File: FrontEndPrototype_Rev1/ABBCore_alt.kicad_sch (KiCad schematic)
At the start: 20 parts, among them J10 MIllMaxSpringConnector, J3 MIllMaxSpringConnector, J4 MIllMaxSpringConnector, J5 MIllMaxSpringConnector, J6 MIllMaxSpringConnector, J7 MIllMaxSpringConnector, J8 MIllMaxSpringConnector, J9 MIllMaxSpringConnector, U1 CD74AC238, U2 ADA4807-2ACP

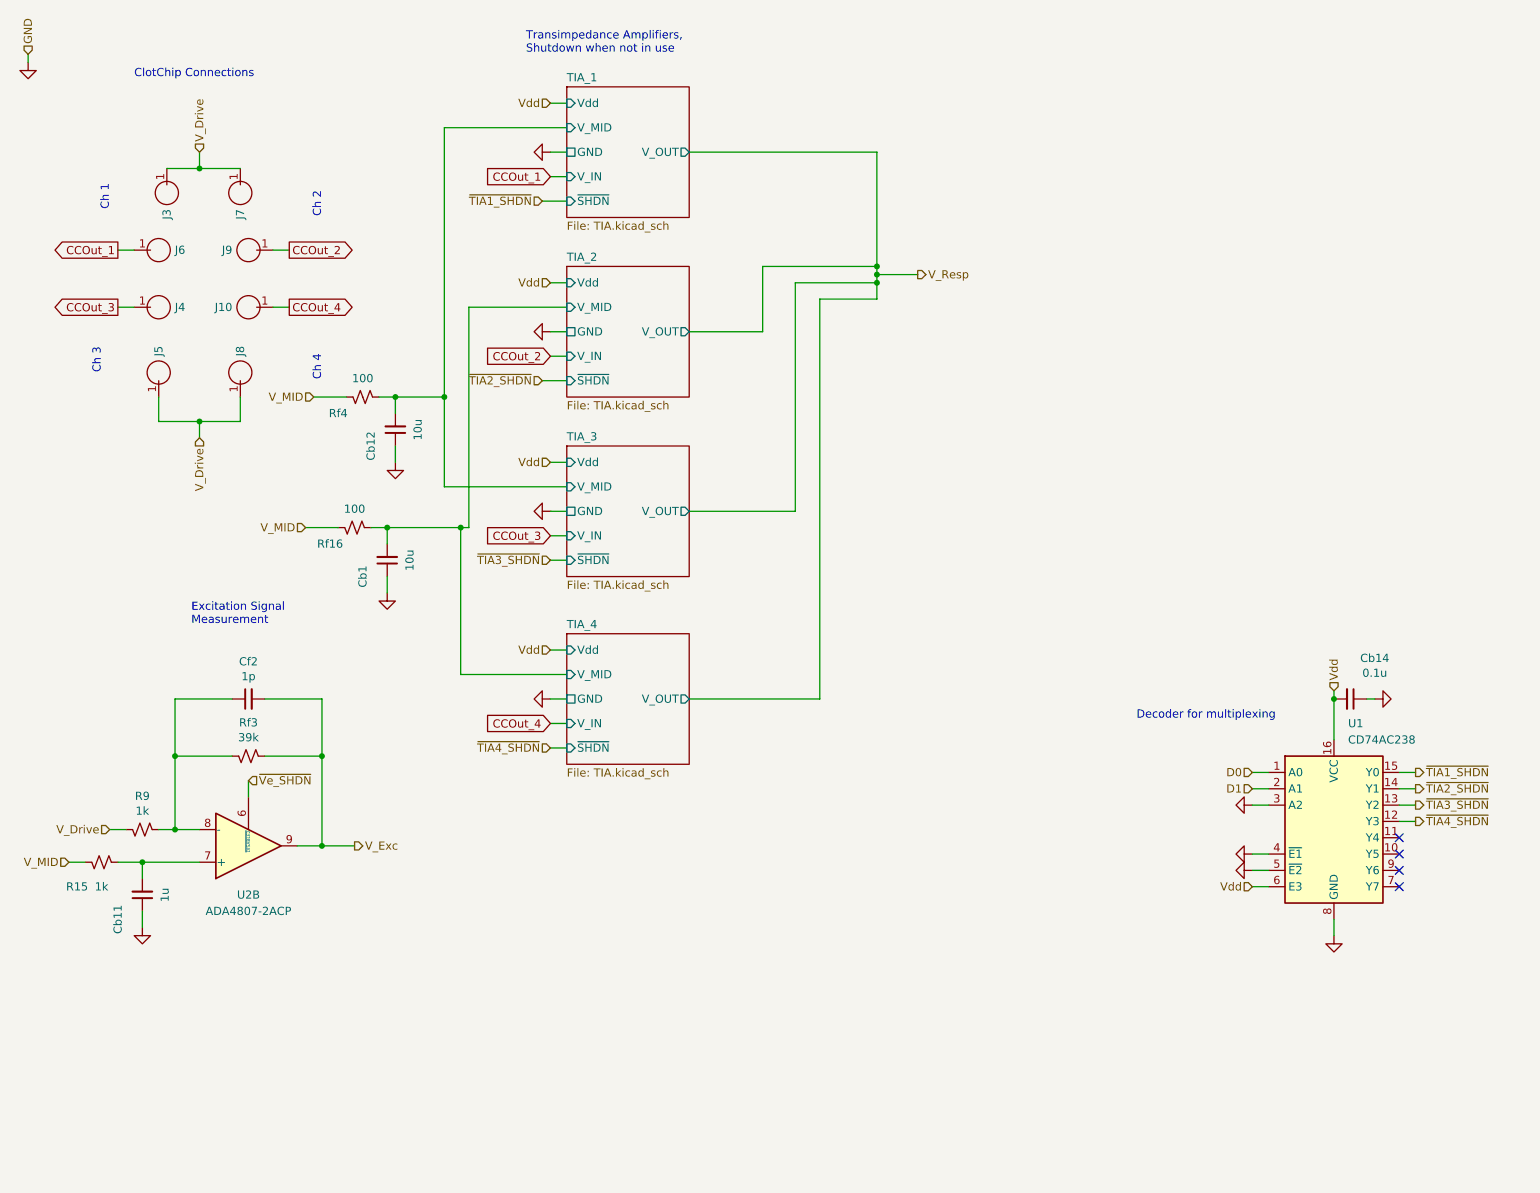
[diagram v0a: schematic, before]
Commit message: First Pass Schematic Fixes for Power Management Board
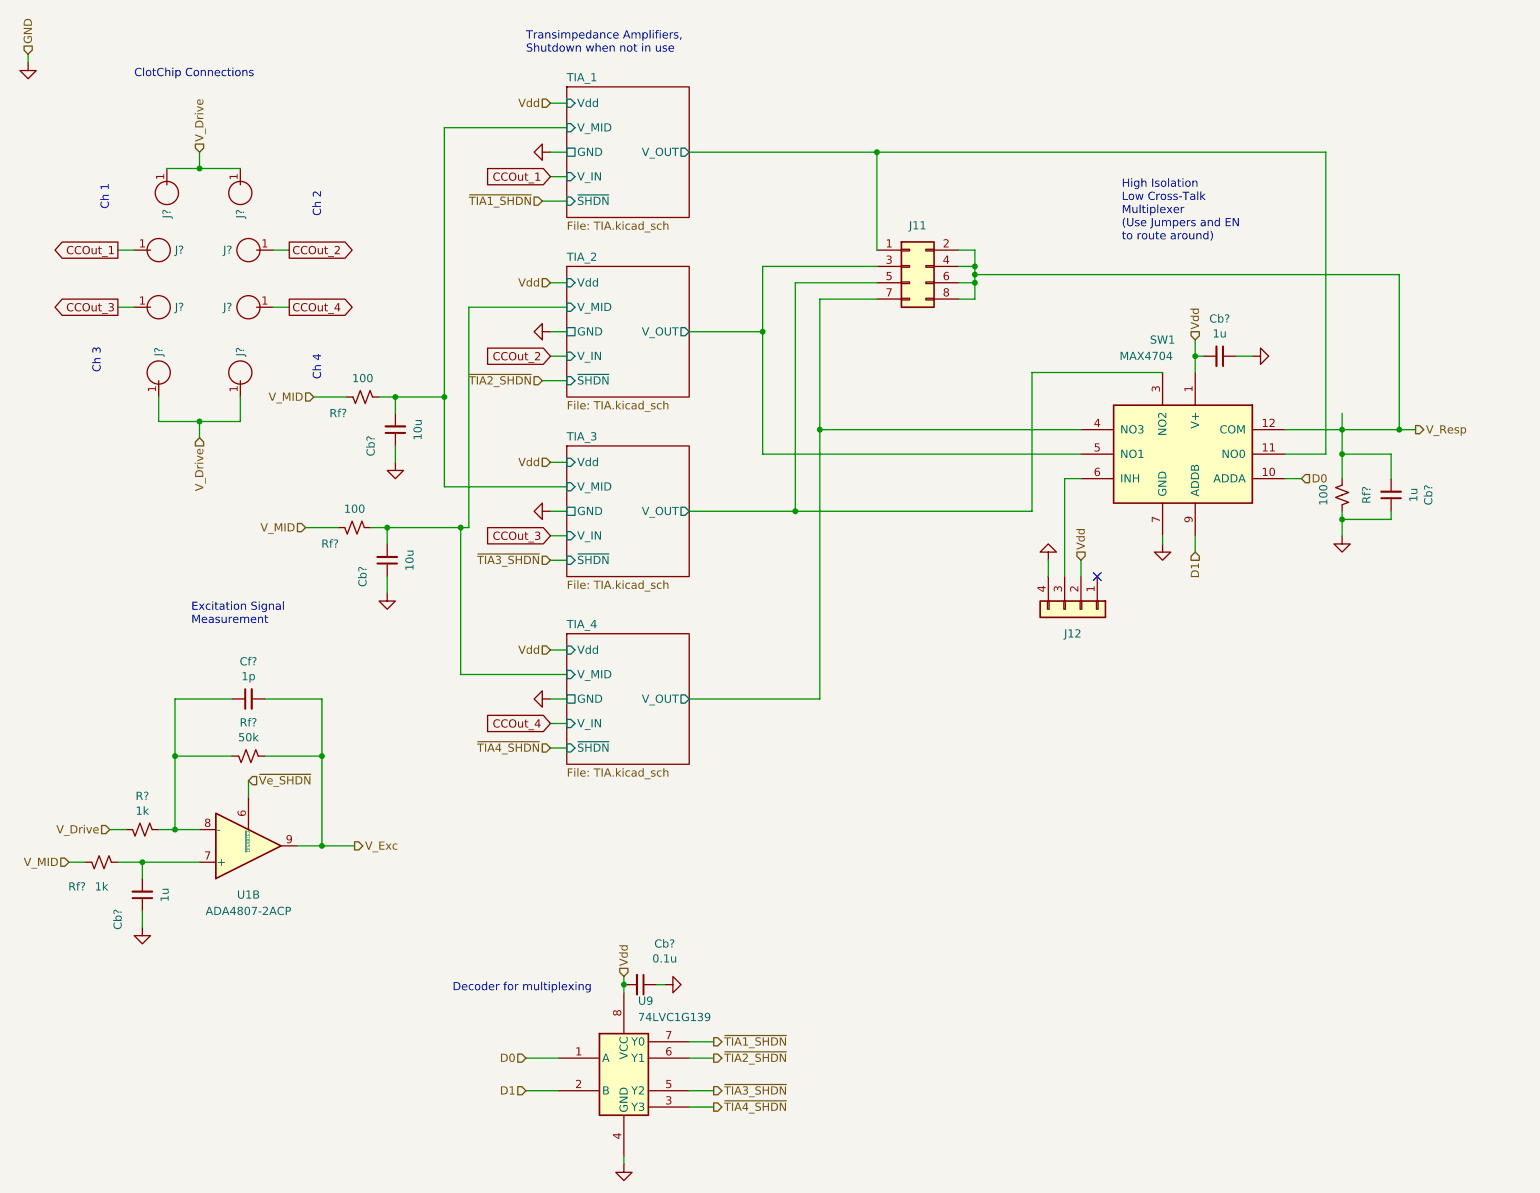
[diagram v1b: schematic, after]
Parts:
- removed Cb14: 0.1u, Capacitor_SMD:C_0603_1608Metric_Pad1.08x0.95mm_HandSolder, symbol Device:C_Small
- removed U1: CD74AC238, Package_SO:TSSOP-16_4.4x5mm_P0.65mm, symbol 74xx:CD74AC238
- added Cb? (x2): 1u, Capacitor_SMD:C_0603_1608Metric_Pad1.08x0.95mm_HandSolder, symbol Device:C_Small
- added Cb?: 0.1u, Capacitor_SMD:C_0603_1608Metric_Pad1.08x0.95mm_HandSolder, symbol Device:C_Small
- added J11: Conn_02x04_Odd_Even, Connector_PinHeader_2.54mm:PinHeader_2x04_P2.54mm_Vertical_SMD, symbol Connector_Generic:Conn_02x04_Odd_Even
- added J12: Conn_02x02_Odd_Even, Connector_PinHeader_2.54mm:PinHeader_1x04_P2.54mm_Vertical_SMD_Pin1Right, symbol Connector_Generic:Conn_01x04
- added Rf?: 100, Resistor_SMD:R_0603_1608Metric_Pad0.98x0.95mm_HandSolder, symbol Device:R_Small_US
- added SW1: MAX4704, Package_DFN_QFN:DFN-12-1EP_3x3mm_P0.5mm_EP1.6x2.5mm, symbol FrontEndPrototype_Rev1-rescue:MAX4704
- added U9: 74LVC1G139, Package_SO:VSSOP-8_2.3x2mm_P0.5mm, symbol 74xGxx:74LVC1G139
- Rf?: renamed from Rf3; value 39k -> 50k
- renumbered Cb11 to Cb?, Cb12 to Cb?, Cb1 to Cb?, Cf2 to Cf?, J9 to J?, J3 to J?, J7 to J?, J5 to J?, J6 to J?, J8 to J?, J10 to J?, J4 to J?, R9 to R?, R15 to Rf?, Rf4 to Rf?, Rf16 to Rf?, U2 to U1
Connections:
- net D0: now also SW1.10 (ADDA), U9.1 (A)
- net D1: now also SW1.9 (ADDB), U9.2 (B)
- net GND: now also Cb?.1, Cb?.1, Cb?.1, J12.4 (Pin_4), Rf?.1, SW1.7 (GND), U9.4 (GND)
- net V_Resp: now also Cb?.2, J11.2 (Pin_2), J11.4 (Pin_4), J11.6 (Pin_6), J11.8 (Pin_8), Rf?.2, SW1.12 (COM)
- net Vdd: now also Cb?.2, Cb?.2, J12.2 (Pin_2), SW1.1 (V+), U9.8 (VCC)
- net ~{TIA1_SHDN}: now also U9.7 (Y0)
- net ~{TIA2_SHDN}: now also U9.6 (Y1)
- net ~{TIA3_SHDN}: now also U9.5 (Y2)
- net ~{TIA4_SHDN}: now also U9.3 (Y3)
- new net: J12.3 (Pin_3), SW1.6 (INH)
- new net TIA_1/V_OUT: J11.1 (Pin_1), SW1.11 (NO0)
- new net TIA_2/V_OUT: J11.3 (Pin_3), SW1.5 (NO1)
- new net TIA_3/V_OUT: J11.5 (Pin_5), SW1.3 (NO2)
- new net TIA_4/V_OUT: J11.7 (Pin_7), SW1.4 (NO3)
- no-connect marks 4 -> 1
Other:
- note added: "High Isolation Low Cross-Talk Multiplexer (Use Jumpers and EN to route around)"

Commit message: Updated Measurement Board with new 3V Reference
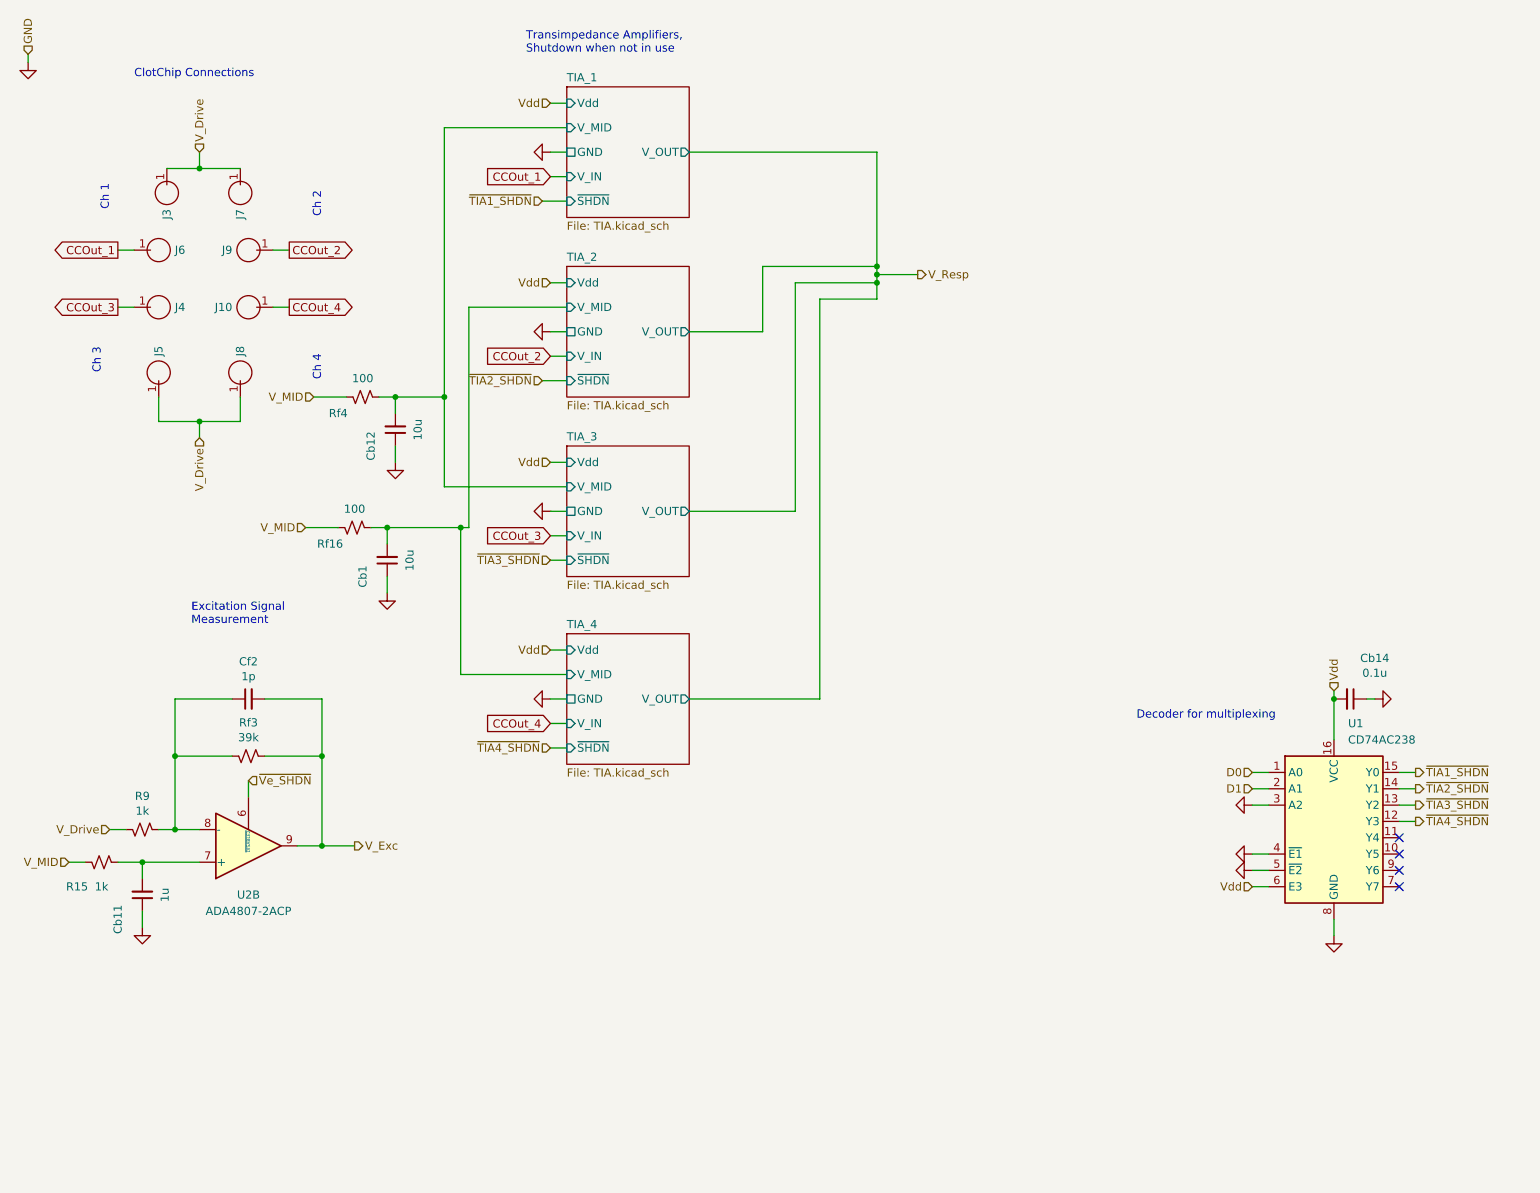
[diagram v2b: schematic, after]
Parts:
- removed Cb? (x2): 1u, Capacitor_SMD:C_0603_1608Metric_Pad1.08x0.95mm_HandSolder, symbol Device:C_Small
- removed Cb?: 0.1u, Capacitor_SMD:C_0603_1608Metric_Pad1.08x0.95mm_HandSolder, symbol Device:C_Small
- removed J11: Conn_02x04_Odd_Even, Connector_PinHeader_2.54mm:PinHeader_2x04_P2.54mm_Vertical_SMD, symbol Connector_Generic:Conn_02x04_Odd_Even
- removed J12: Conn_02x02_Odd_Even, Connector_PinHeader_2.54mm:PinHeader_1x04_P2.54mm_Vertical_SMD_Pin1Right, symbol Connector_Generic:Conn_01x04
- removed Rf?: 100, Resistor_SMD:R_0603_1608Metric_Pad0.98x0.95mm_HandSolder, symbol Device:R_Small_US
- removed SW1: MAX4704, Package_DFN_QFN:DFN-12-1EP_3x3mm_P0.5mm_EP1.6x2.5mm, symbol FrontEndPrototype_Rev1-rescue:MAX4704
- removed U9: 74LVC1G139, Package_SO:VSSOP-8_2.3x2mm_P0.5mm, symbol 74xGxx:74LVC1G139
- added Cb14: 0.1u, Capacitor_SMD:C_0603_1608Metric_Pad1.08x0.95mm_HandSolder, symbol Device:C_Small
- added U1: CD74AC238, Package_SO:TSSOP-16_4.4x5mm_P0.65mm, symbol 74xx:CD74AC238
- Rf3: renamed from Rf?; value 50k -> 39k
- gave numbers to parts that had none: 16
- renumbered U1 to U2
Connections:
- net D0: now also U1.1 (A0)
- net D1: now also U1.2 (A1)
- net GND: now also Cb14.1, U1.3 (A2), U1.4 (~{E1}), U1.5 (~{E2}), U1.8 (GND)
- net Vdd: now also Cb14.2, U1.16 (VCC), U1.6 (E3)
- net ~{TIA1_SHDN}: now also U1.15 (Y0)
- net ~{TIA2_SHDN}: now also U1.14 (Y1)
- net ~{TIA3_SHDN}: now also U1.13 (Y2)
- net ~{TIA4_SHDN}: now also U1.12 (Y3)
- no-connect marks 1 -> 4
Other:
- note removed: "High Isolation Low Cross-Talk Multiplexer (Use Jumpers and EN to route around)"
